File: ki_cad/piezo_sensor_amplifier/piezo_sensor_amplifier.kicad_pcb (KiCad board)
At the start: 2 copper layers, 24.9 x 24.9 mm, 12 parts, among them J1 Conn_01x03, U1 MCP6476T-E/OT, Y1 Piezo Sensor 40kHz

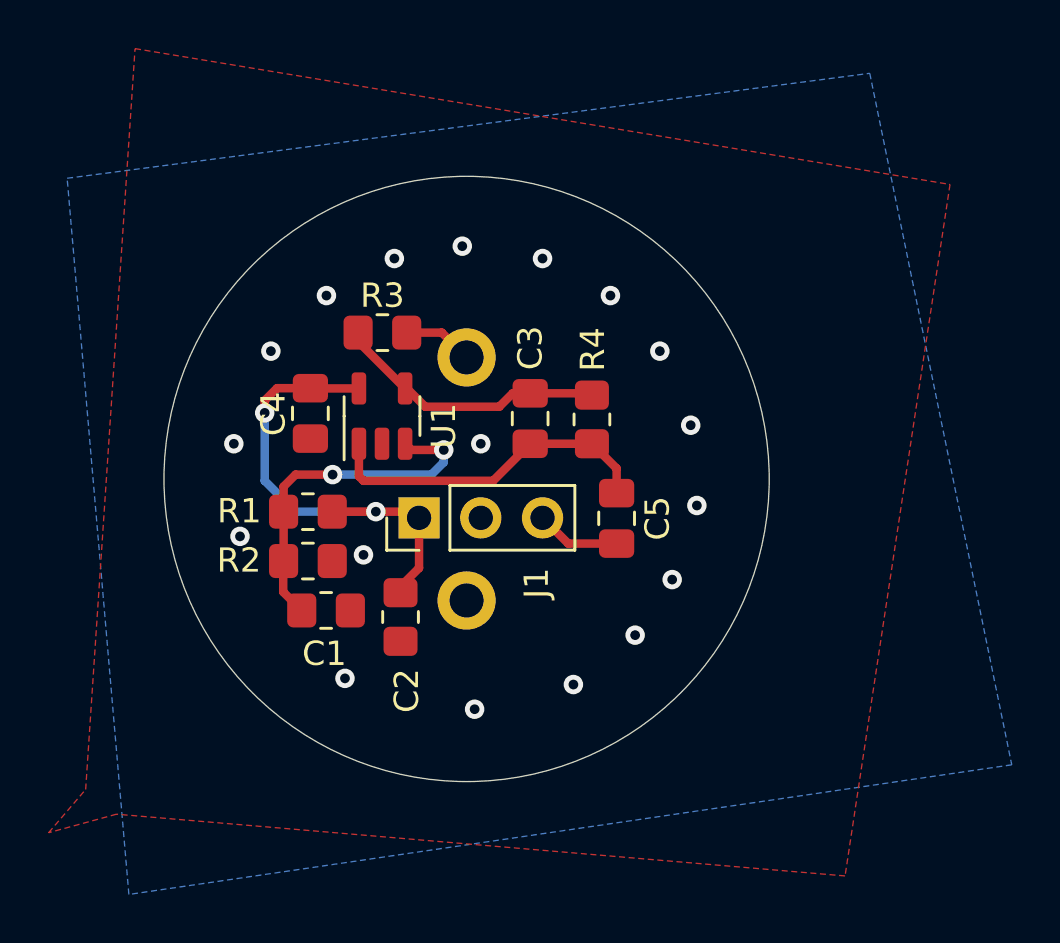
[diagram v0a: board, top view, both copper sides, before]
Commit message: first working hardware board :)
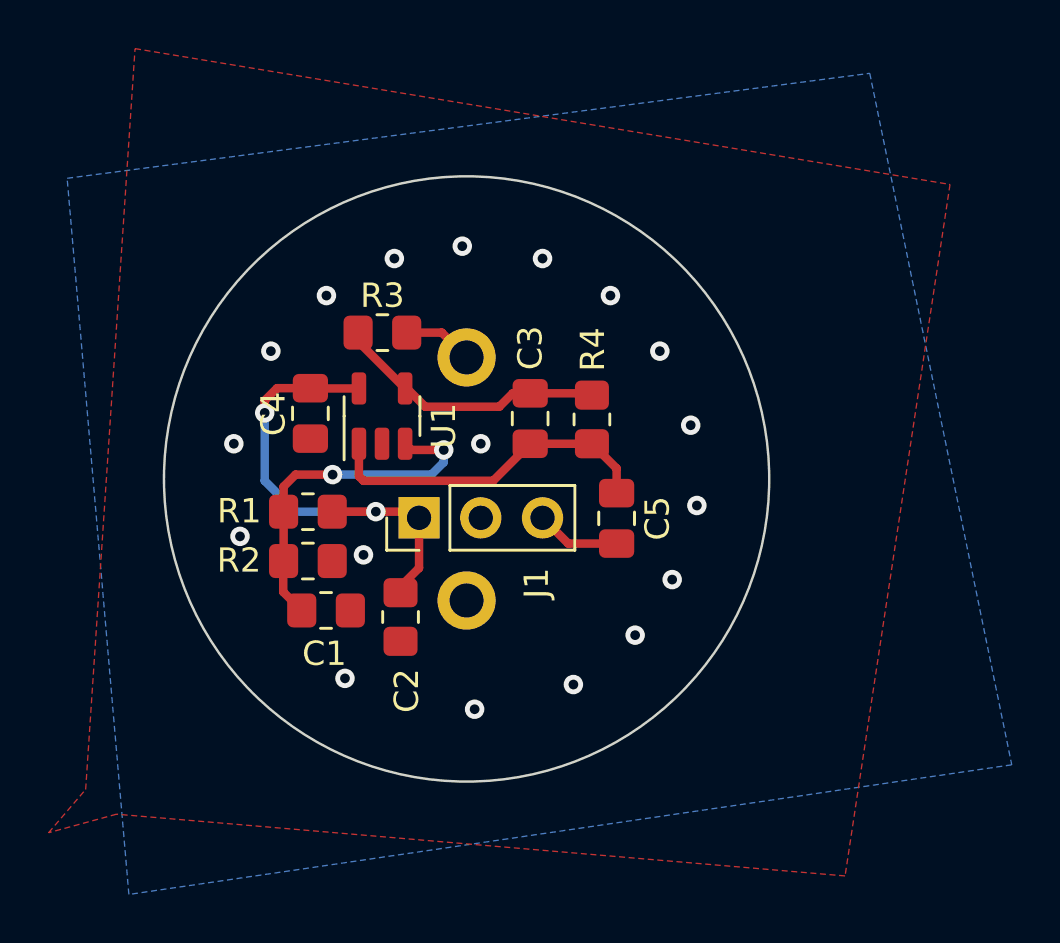
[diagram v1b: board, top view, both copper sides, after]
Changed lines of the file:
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@@
       (effects (font (size 1 1) (thickness 0.15)))
     )
-    (fp_text value "33p" (at -0.2 1.45 90) (layer "F.Fab")
+    (fp_text value "33p" (at -3.4395 -0.059 90) (layer "F.Fab")
       (effects (font (size 1 1) (thickness 0.15)))
     )
@@
       (effects (font (size 1 1) (thickness 0.15)) (justify mirror))
     )
-    (fp_text value "Piezo Sensor 40kHz" (at 0 0 unlocked) (layer "F.Fab")
+    (fp_text value "Piezo Sensor 40kHz" (at -0.55 11.35 unlocked) (layer "F.Fab")
       (effects (font (size 1 1) (thickness 0.15)))
     )
@@
       (effects (font (size 1 1) (thickness 0.15)))
     )
-    (fp_text value "20k" (at 0 1.65) (layer "F.Fab")
+    (fp_text value "20k" (at -3.222 -0.028) (layer "F.Fab")
       (effects (font (size 1 1) (thickness 0.15)))
     )
@@
       (effects (font (size 1 1) (thickness 0.15)))
     )
-    (fp_text value "Conn_01x03" (at 0 7.41 90) (layer "F.Fab")
+    (fp_text value "Conn_01x03" (at 0 7.41 90) (layer "F.Fab") hide
       (effects (font (size 1 1) (thickness 0.15)))
     )
@@
       (effects (font (size 1 1) (thickness 0.15)))
     )
-    (fp_text value "1u" (at 0.03 -0.012 90) (layer "F.Fab")
+    (fp_text value "1u" (at 2.92 0.107 90) (layer "F.Fab")
       (effects (font (size 1 1) (thickness 0.15)))
     )
@@
       (effects (font (size 1 1) (thickness 0.15)))
     )
-    (fp_text value "1u" (at 0.01 0.136) (layer "F.Fab")
+    (fp_text value "1u" (at 0.007 1.815) (layer "F.Fab")
       (effects (font (size 1 1) (thickness 0.15)))
     )
@@
       (effects (font (size 1 1) (thickness 0.15)))
     )
-    (fp_text value "10n" (at 0 1.68 90) (layer "F.Fab")
+    (fp_text value "10n" (at 0.0535 -1.853 90) (layer "F.Fab")
       (effects (font (size 1 1) (thickness 0.15)))
     )
@@
       (effects (font (size 1 1) (thickness 0.15)))
     )
-    (fp_text value "1MEG" (at 0 1.65 90) (layer "F.Fab")
+    (fp_text value "1MEG" (at -4.002 -0.144 90) (layer "F.Fab")
       (effects (font (size 1 1) (thickness 0.15)))
     )
@@
       (effects (font (size 1 1) (thickness 0.15)))
     )
-    (fp_text value "20k" (at 0 1.65) (layer "F.Fab")
+    (fp_text value "20k" (at 3.347 0.096) (layer "F.Fab")
       (effects (font (size 1 1) (thickness 0.15)))
     )
@@
       (effects (font (size 1 1) (thickness 0.15)))
     )
-    (fp_text value "MCP6476T-E/OT" (at 0 2.4 90) (layer "F.Fab")
+    (fp_text value "MCP6476T-E/OT" (at -0.4855 -10.695 90) (layer "F.Fab")
       (effects (font (size 1 1) (thickness 0.15)))
     )
@@
     )
   )
-  (gr_circle locked (center 100 100) (end 112.45 100) (layer "Edge.Cuts") (width 0) (fill none))
+  (gr_circle locked (center 100 100) (end 112.45 100) (layer "Edge.Cuts") (width 0.1) (fill none))
   (gr_circle locked (center 100 100) (end 110 100) (layer "F.Fab") (width 0.1) (fill none))
   (segment (start 93.218 105.41) (end 92.456 104.648) (width 0.35) (layer "F.Cu") (net 1))
